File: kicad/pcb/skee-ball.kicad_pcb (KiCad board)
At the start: 2 copper layers, 65 parts, among them J1 SPEAKER, J11 NHD_DB1, J12 NHD_DB0, J13 HEADER, J18 DC_DRIVER, J19 JOYSTICK, J2 EXTERNAL_BUTTON, J20 SERVO, J21 US0, J22 US1, J23 NHD_E1, J24 NHD_E2, J26 US2, J27 US3, J3 Conn_02x06_Counter_Clockwise, J36 US4, J4 Barrel_Jack, J9 NHD_RS, SW1 SW_Push, U1 D24V22F6, U13 LD1117S33TR_SOT223, U2 MAX98357A, U3 D24V22F5, U4 STM32F091RCTx, U5 74HC595, U6 74HC595, U7 74LS08

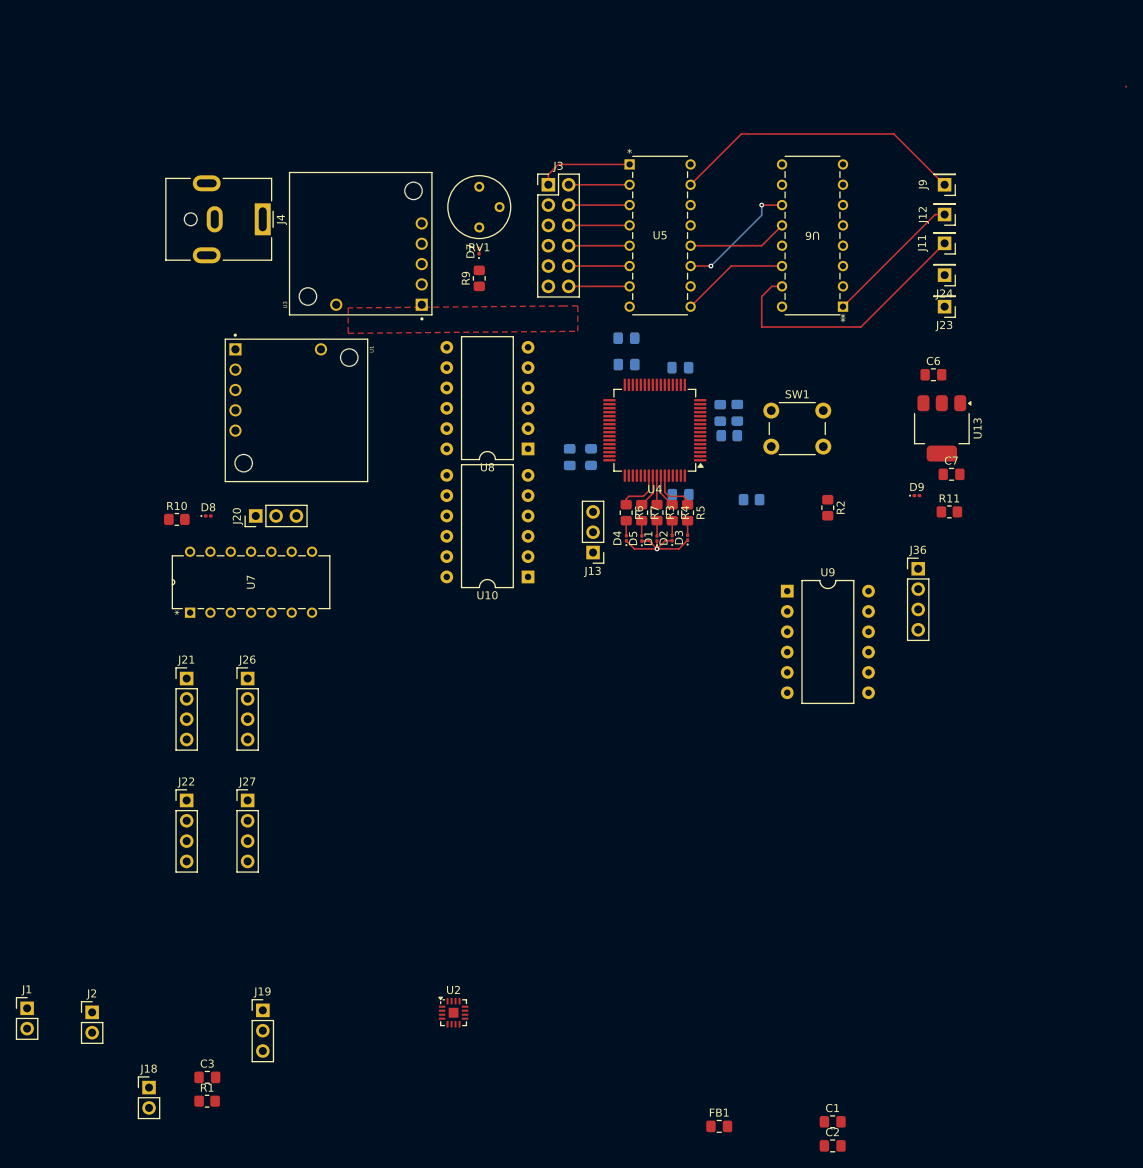
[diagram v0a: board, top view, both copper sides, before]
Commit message: finish routing
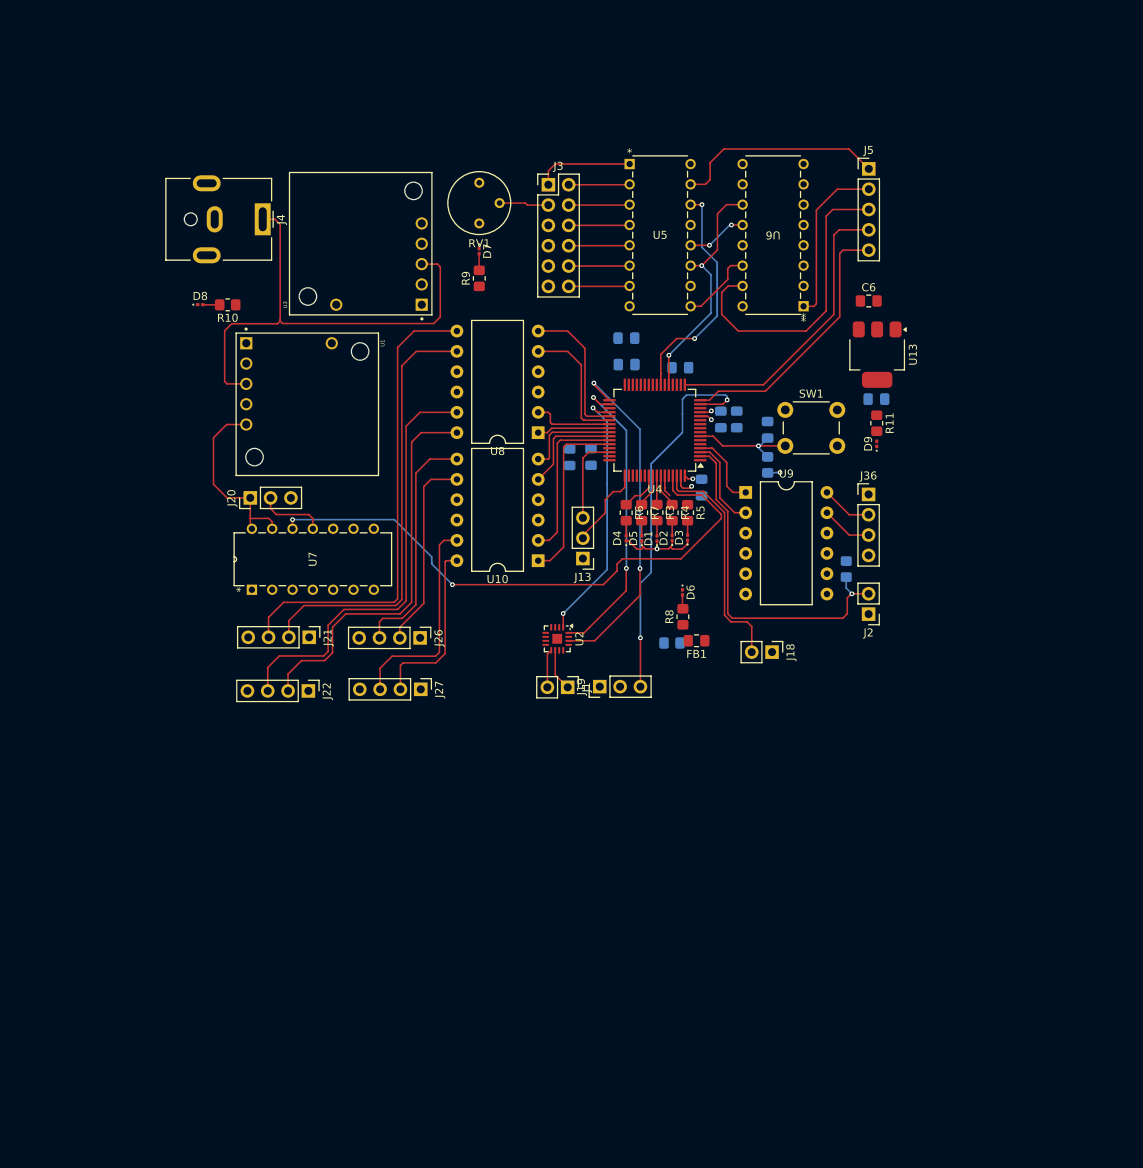
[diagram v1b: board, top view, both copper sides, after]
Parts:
- removed C18: 10nF, Capacitor_SMD:C_0805_2012Metric_Pad1.18x1.45mm_HandSolder
- removed C19: 1uF, Capacitor_SMD:C_0805_2012Metric_Pad1.18x1.45mm_HandSolder
- removed J11: NHD_DB1, Connector_PinHeader_2.54mm:PinHeader_1x01_P2.54mm_Vertical
- removed J12: NHD_DB0, Connector_PinHeader_2.54mm:PinHeader_1x01_P2.54mm_Vertical
- removed J23: NHD_E1, Connector_PinHeader_2.54mm:PinHeader_1x01_P2.54mm_Vertical
- removed J24: NHD_E2, Connector_PinHeader_2.54mm:PinHeader_1x01_P2.54mm_Vertical
- removed J9: NHD_RS, Connector_PinHeader_2.54mm:PinHeader_1x01_P2.54mm_Vertical
- removed the R1 at (79.3, 156.5)
- removed the R1 at (144.5, 73.3)
- added D6: LED, LED_SMD:LED_0201_0603Metric, F.Cu at (138.7, 92.9)
- added J5: Conn_01x05, Connector_PinHeader_2.54mm:PinHeader_1x05_P2.54mm_Vertical, F.Cu at (162.0, 39.9)
- added R1: 10k, Resistor_SMD:R_0805_2012Metric_Pad1.20x1.40mm_HandSolder, B.Cu at (149.3, 76.9)
- added R8: 150, Resistor_SMD:R_0805_2012Metric_Pad1.20x1.40mm_HandSolder, F.Cu at (138.7, 95.9)
- C1, C2, C3, C7, R2: moved to B.Cu
- R10: value 150 -> 300
- R9: value 150 -> 200
- moved J2 109.1 mm to (162.0, 95.6), turned to 180 degrees
- moved C3 107.0 mm to (149.3, 72.5), turned to -90 degrees
- moved J18 95.0 mm to (149.9, 100.3), turned to -90 degrees
- moved C2 91.6 mm to (145.5, 71.2), turned to -90 degrees
- moved C1 88.9 mm to (143.5, 71.2), turned to -90 degrees
- moved J1 78.6 mm to (124.3, 104.7), turned to -90 degrees
- moved FB1 60.8 mm to (140.4, 98.9), turned to 180 degrees
- moved J19 58.4 mm to (128.4, 104.6), turned to 90 degrees
- moved U2 48.5 mm to (123.0, 98.7), turned to -90 degrees
- moved R10 27.6 mm to (81.8, 56.9), turned to 180 degrees
- moved D8 26.4 mm to (78.4, 56.9)
- moved J27 25.7 mm to (106.0, 105.0), turned to -90 degrees
- moved J26 22.2 mm to (105.9, 98.6), turned to -90 degrees
- moved R12 20.5 mm to (137.4, 99.2)
- moved J22 20.5 mm to (91.9, 105.2), turned to -90 degrees
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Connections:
- J13 pad 1: SWCLK -> GND
- J13 pad 2: SWDIO -> SWCLK
- J13 pad 3: GND -> SWDIO
- J20 pad 1: PWM_SERVO_6 -> +6V
- J20 pad 2: +6V -> PWM_SERVO_6
- U2 pad 7: VDD -> VDA
- U2 pad 8: VDD -> VDA
- U4 pad 3: US_TRIG4_3.3 -> US_ECHO4_3.3
- U4 pad 4: US_ECHO4_3.3 -> US_TRIG4_3.3
- U9 pad 1: unconnected-(U9-LV4-Pad1) -> US_TRIG4_3.3
- U9 pad 11: unconnected-(U9-HV3-Pad11) -> US_ECHO4_5
- U9 pad 12: unconnected-(U9-HV4-Pad12) -> US_TRIG4_5
- U9 pad 2: unconnected-(U9-LV3-Pad2) -> US_ECHO4_3.3
- U9 pad 5: US_TRIG4_3.3 -> unconnected-(U9-LV2-Pad5)
- U9 pad 6: US_ECHO4_3.3 -> unconnected-(U9-LV1-Pad6)
- U9 pad 7: US_ECHO4_5 -> unconnected-(U9-HV1-Pad7)
- U9 pad 8: US_TRIG4_5 -> unconnected-(U9-HV2-Pad8)
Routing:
- net PWM_SERVO_3.3: track 0.00 -> 72.3 mm, vias 0 -> 2
- net +24V: track 0.00 -> 60.3 mm
- net US_ECHO0_5: track 0.00 -> 59.3 mm
- net US_ECHO1_5: track 0.00 -> 54.5 mm
- net US_TRIG0_5: track 0.00 -> 54.2 mm
- net US_TRIG1_5: track 0.00 -> 49.3 mm
- net ADC_IN1: track 0.00 -> 48.0 mm, vias 0 -> 2
- net BUTTON_IN: track 0.00 -> 44.4 mm, vias 0 -> 1
- net SPI2-NSS(I2S_WS): track 0.00 -> 43.1 mm, vias 0 -> 2
- net NHD_DB1: track 0.00 -> 38.2 mm
- net SPI2-SCK(I2S_CK): track 0.00 -> 37.6 mm, vias 0 -> 2
- net Net-(J9-Pin_1): track 37.0 -> 0.00 mm
- net NHD_E2: track 0.00 -> 36.8 mm
- net Net-(J11-Pin_1): track 34.1 -> 0.00 mm
- net NHD_E1: track 0.00 -> 33.5 mm
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- removed copper zone on F.Cu, net +5V

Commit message: created version 8.0 of pcb
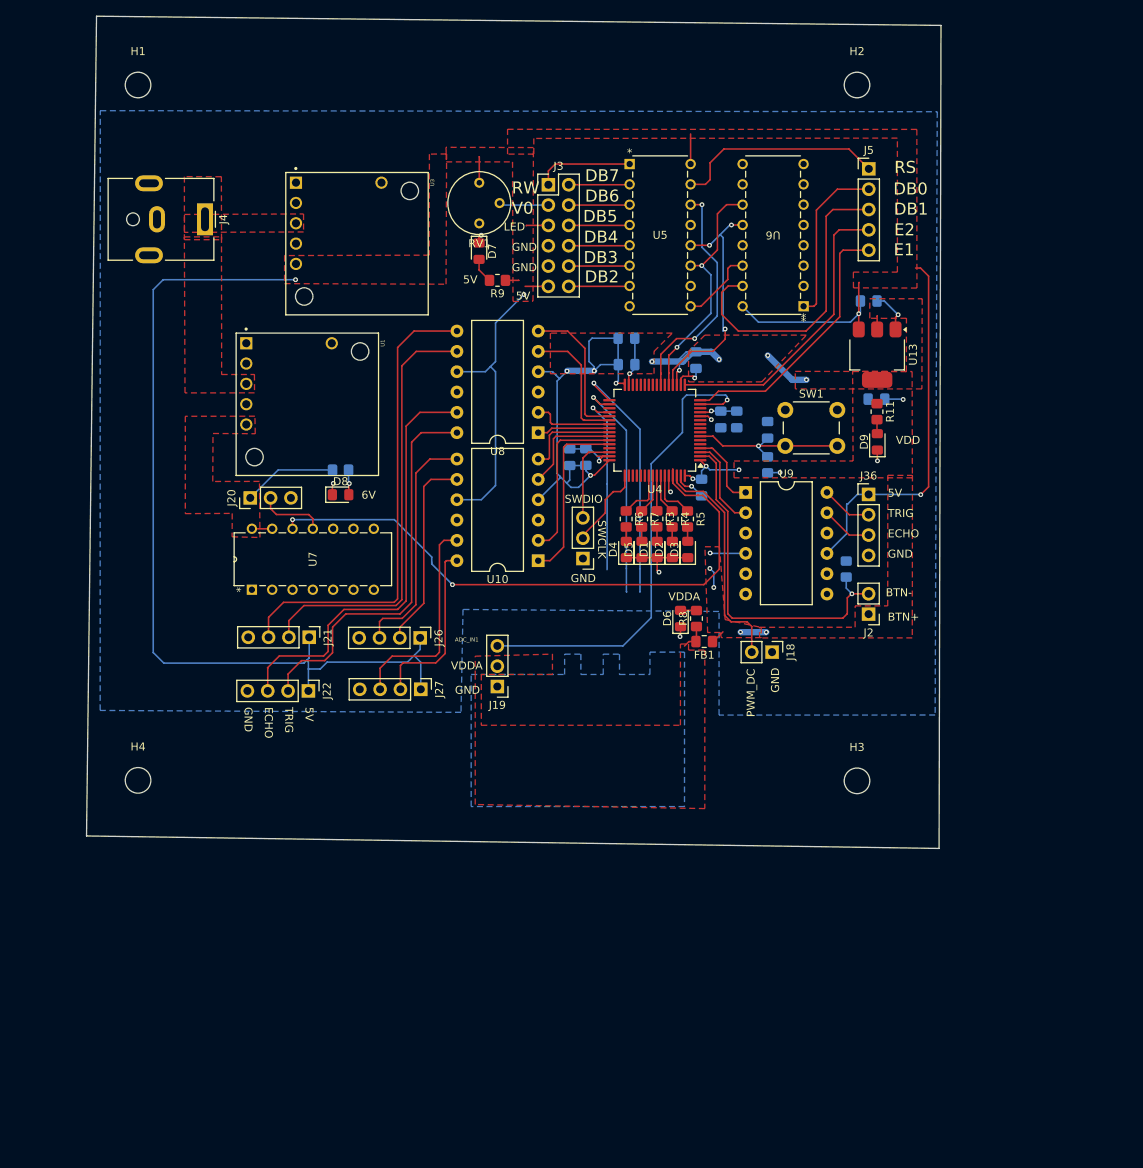
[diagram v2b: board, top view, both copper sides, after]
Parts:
- removed J1: SPEAKER, Connector_PinHeader_2.54mm:PinHeader_1x02_P2.54mm_Vertical
- removed R12: 0, Resistor_SMD:R_0805_2012Metric_Pad1.20x1.40mm_HandSolder
- removed U2: MAX98357A, Package_DFN_QFN:TQFN-16-1EP_3x3mm_P0.5mm_EP1.23x1.23mm
- added H1: MountingHole, MountingHole:MountingHole_3.2mm_M3, F.Cu at (70.6, 29.4)
- added H2: MountingHole, MountingHole:MountingHole_3.2mm_M3, F.Cu at (160.5, 29.4)
- added H3: MountingHole, MountingHole:MountingHole_3.2mm_M3, F.Cu at (160.5, 116.4)
- added H4: MountingHole, MountingHole:MountingHole_3.2mm_M3, F.Cu at (70.6, 116.4)
- C6, R10: moved to B.Cu
- D1, D2, D3, D4, D5, D6, D7, D8, D9: footprint LED_SMD:LED_0201_0603Metric -> LED_SMD:LED_0805_2012Metric_Pad1.15x1.40mm_HandSolder
- moved D8 29.5 mm to (96.0, 80.7)
- moved R10 25.0 mm to (95.9, 77.6), turned to 0 degrees
- moved J19 12.8 mm to (115.5, 104.6), turned to 180 degrees
- moved J4 7.22 mm to (79.0, 46.2)
- moved D6 3.28 mm to (138.4, 96.1), turned to 90 degrees
- moved R9 2.29 mm to (115.6, 53.9), turned to 180 degrees
- moved C10 2.17 mm to (140.4, 63.8), turned to -90 degrees
- moved R8 1.71 mm to (140.4, 96.1)
- moved D3 1.48 mm to (139.3, 87.5)
- moved R11 1.45 mm to (163.0, 70.3)
- moved D2 1.42 mm to (137.4, 87.5)
- moved D4 1.40 mm to (131.7, 87.5)
- moved D5 1.38 mm to (133.6, 87.5)
- moved D1 1.38 mm to (135.5, 87.5)
- moved FB1 0.96 mm to (141.4, 99.0)
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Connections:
- J19 pad 2: VDA -> VDDA
- R8 pad 1: VDA -> VDDA
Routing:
- net +5V: track 0.00 -> 231.8 mm, vias 0 -> 4
- net VDD: track 2.82 -> 105.3 mm, vias 2 -> 19
- net +24V: track 60.3 -> 0.00 mm
- net GND: track 14.8 -> 44.2 mm, vias 2 -> 11
- net RCLK: track 7.55 -> 31.4 mm, vias 2 -> 3
- net SPI2-NSS(I2S_WS): track 43.1 -> 31.4 mm, vias 2 -> 1
- net ADC_IN1: track 48.0 -> 59.5 mm, vias 2 -> 1
- net SPI2-MOSI(I2S_SD): track 32.8 -> 23.3 mm, vias 2 -> 1
- net SPI2-SCK(I2S_CK): track 37.6 -> 28.4 mm, vias 2 -> 1
- net +6V: track 23.6 -> 14.6 mm
- net VDDA: track 1.46 -> 8.21 mm
- net NRST: track 14.6 -> 21.1 mm
- net Net-(J1-Pin_1): track 5.26 -> 0.00 mm
- net Net-(J1-Pin_2): track 4.82 -> 0.00 mm
- net PWM_SERVO_3.3: track 72.3 -> 76.4 mm
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- added copper zone on F.Cu, net +24V
- added copper zone on F.Cu, net +5V
- added copper zone on F.Cu, net +6V
- added copper zone on B.Cu, net GND
- added copper zone on F.Cu, net VDD
- added copper zone on F.Cu, net VDDA
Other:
- board outline added: 106.8 x 104 mm
- board text added: "5V"
- board text added: "6V"
- board text added: "ADC_IN1"
- board text added: "BTN+"
- board text added: "BTN-"
- board text added: "DB0"
- board text added: "DB1"
- board text added: "DB2"
- board text added: "DB3"
- board text added: "DB4"
- board text added: "DB5"
- board text added: "DB6"
- board text added: "DB7"
- board text added: "David Fall Andrew Cali Jennifer Ferguson Madeline Flanagan"
- board text added: "E1"
- board text added: "E2"
- board text added: "ECE 47700 Team #1 Electronic Skee Ball Spring 2025"
- board text added: "ECHO"
- board text added: "GND"
- board text added: "LED"
- board text added: "PWM_DC"
- board text added: "RS"
- board text added: "RW"
- board text added: "SWCLK"
- board text added: "SWDIO"
- board text added: "TRIG"
- board text added: "V0"
- board text added: "VDD"
- board text added: "VDDA"
